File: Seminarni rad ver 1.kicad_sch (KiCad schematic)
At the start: 35 parts, among them J1 Screw_Terminal_01x02 (Izlaz), J2 Screw_Terminal_01x02(power), J3 Screw_Terminal_01x02(ulaz), Q1 IRLZ44N, Q4 2N7000, SW1 SW_Nidec_CAS-120A1, U2 NE555P, U3 DL1416, U4 ATtiny3217-M, U5 INA260, X7RDielectric2 100n

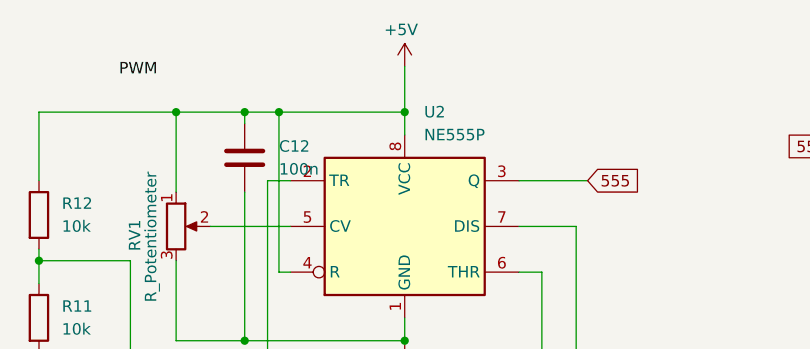
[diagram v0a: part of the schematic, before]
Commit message: chande
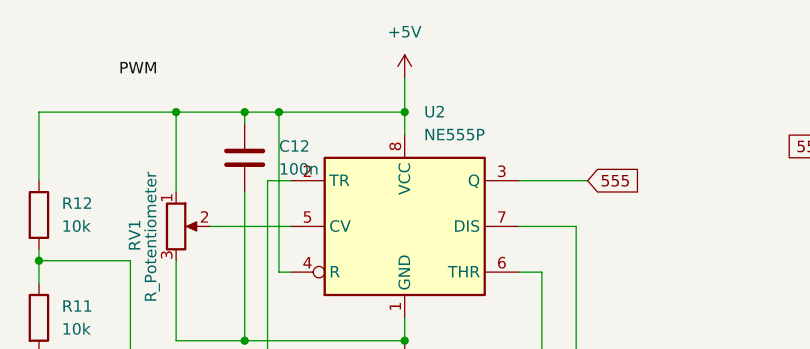
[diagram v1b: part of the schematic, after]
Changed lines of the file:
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@@
 	)
 	(junction
-		(at 139.7 50.8)
+		(at 59.69 22.86)
 		(diameter 0)
 		(color 0 0 0 0)
 	)
 	(junction
-		(at 59.69 22.86)
+		(at 139.7 50.8)
 		(diameter 0)
 		(color 0 0 0 0)
@@
 	(wire
 		(pts
-			(xy 59.69 17.78) (xy 59.69 22.86)
-		)
-		(stroke
-			(width 0)
-			(type default)
-		)
-	)
-	(wire
-		(pts
 			(xy 187.96 152.4) (xy 187.96 154.94)
 		)
@@
 	(wire
 		(pts
+			(xy 59.69 19.05) (xy 59.69 22.86)
+		)
+		(stroke
+			(width 0)
+			(type default)
+		)
+	)
+	(wire
+		(pts
 			(xy 241.3 149.86) (xy 241.3 151.13)
 		)
@@
 	)
 	(symbol
+		(lib_id "power:+5V")
+		(at 59.69 19.05 0)
+		(unit 1)
+		(exclude_from_sim no)
+		(in_bom yes)
+		(on_board yes)
+		(dnp no)
+		(fields_autoplaced yes)
+		(property "Reference" "#PWR01"
+			(at 59.69 22.86 0)
+			(effects
+				(font
+					(size 1.27 1.27)
+				)
+				(hide yes)
+			)
+		)
+		(property "Value" "+5V"
+			(at 59.69 13.97 0)
+			(effects
+				(font
+					(size 1.27 1.27)
+				)
+			)
+		)
+		(property "Footprint" ""
+			(at 59.69 19.05 0)
+			(effects
+				(font
+					(size 1.27 1.27)
+				)
+				(hide yes)
+			)
+		)
+		(property "Datasheet" ""
+			(at 59.69 19.05 0)
+			(effects
+				(font
+					(size 1.27 1.27)
+				)
+				(hide yes)
+			)
+		)
+		(property "Description" "Power symbol creates a global label with name \"+5V\""
+			(at 59.69 19.05 0)
+			(effects
+				(font
+					(size 1.27 1.27)
+				)
+				(hide yes)
+			)
+		)
+		(pin "1"
+		)
+		(instances
+			(project "Seminarni rad ver 1"
+				(path "/071dfc4d-d3f6-4752-9a76-11410e80c51a"
+					(reference "#PWR01")
+					(unit 1)
+				)
+			)
+		)
+	)
+	(symbol
 		(lib_id "power:GND")
 		(at 29.21 102.87 0)
@@
 					(unit 1)
 				)
-			)
-		)
-	)
-	(symbol
-		(lib_id "power:+5V")
-		(at 59.69 17.78 0)
-		(unit 1)
-		(exclude_from_sim no)
-		(in_bom yes)
-		(on_board yes)
-		(dnp no)
-		(property "Reference" "#PWR01"
-			(at 59.69 21.59 0)
-			(effects
-				(font
-					(size 1.27 1.27)
-				)
-				(hide yes)
-			)
-		)
-		(property "Value" "+5V"
-			(at 57.404 13.716 0)
-			(effects
-				(font
-					(size 1.27 1.27)
-				)
-				(justify left)
-			)
-		)
-		(property "Footprint" ""
-			(at 59.69 17.78 0)
-			(effects
-				(font
-					(size 1.27 1.27)
-				)
-				(hide yes)
-			)
-		)
-		(property "Datasheet" ""
-			(at 59.69 17.78 0)
-			(effects
-				(font
-					(size 1.27 1.27)
-				)
-				(hide yes)
-			)
-		)
-		(property "Description" "Power symbol creates a global label with name \"+5V\""
-			(at 59.69 17.78 0)
-			(effects
-				(font
-					(size 1.27 1.27)
-				)
-				(hide yes)
-			)
-		)
-		(pin "1"
-		)
-		(instances
-			(project ""
-				(path "/071dfc4d-d3f6-4752-9a76-11410e80c51a"
-					(reference "#PWR01")
-					(unit 1)
-				)
